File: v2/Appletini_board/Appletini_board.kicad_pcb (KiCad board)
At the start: 4 copper layers, 152.4 x 69.8 mm, 32 parts, among them J1 Conn_02x25_Counter_Clockwise, Q1 TP0610T, U1 SN74LVC543ADW, U10 SN74LVC543ADW, U14 74AHC1G126, U2 Pico, U3 Teensy4.1, U4 SN74LVC543ADW, U5 TXS0108EPW, U6 74LS08, U7 74AHC1G126, U8 SN74LVC1G14DBV, U9 SN74LVC543ADW

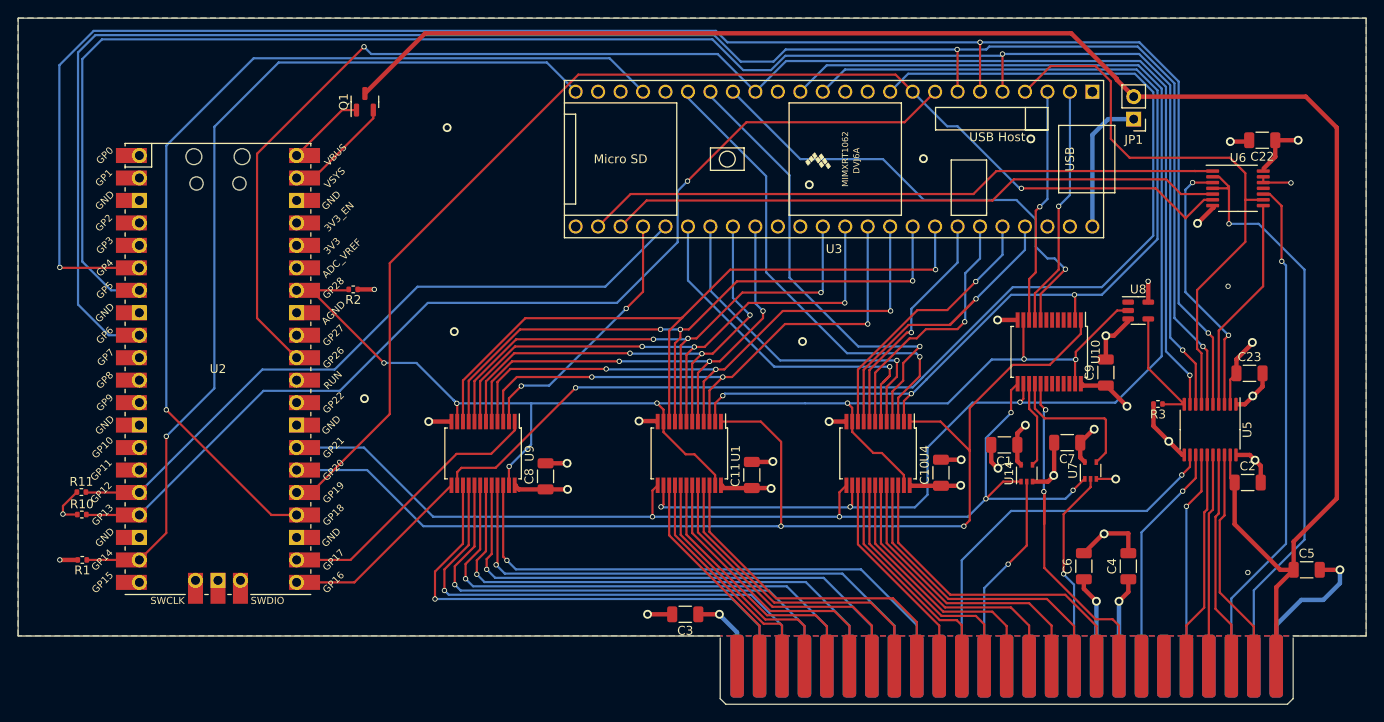
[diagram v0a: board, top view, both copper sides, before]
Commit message: fixes
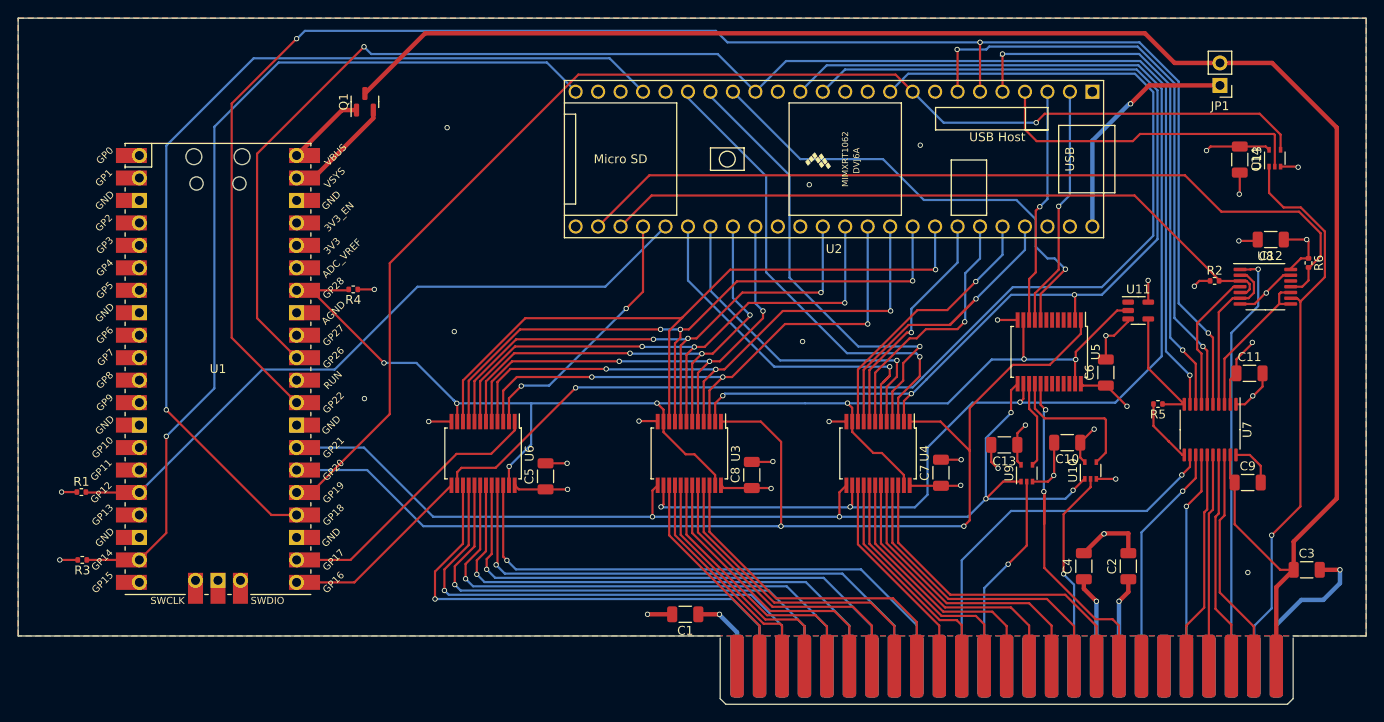
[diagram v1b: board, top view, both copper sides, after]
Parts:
- removed R10: 10K, Resistor_SMD:R_0402_1005Metric
- removed the U6 at (187.9, 69.2)
- added C14: 100pF, Capacitor_SMD:C_1206_3216Metric, F.Cu at (188.1, 66.0)
- added R2: 10K, Resistor_SMD:R_0402_1005Metric, F.Cu at (185.3, 79.7)
- added R6: 10K, Resistor_SMD:R_0402_1005Metric, F.Cu at (195.9, 77.7)
- added U13: 74LVC1G08, Package_TO_SOT_SMD:SOT-353_SC-70-5, F.Cu at (192.1, 65.8)
- added U8: 74LCX07, Package_SO:TSSOP-14_4.4x5mm_P0.65mm, F.Cu at (191.0, 80.4)
- moved C12 11.3 mm to (191.6, 75.0)
- moved JP1 10.5 mm to (185.9, 57.6)
- renumbered C3 to C1, C7 to C10, C23 to C11, C22 to C12, C1 to C13, C4 to C2, C5 to C3, C6 to C4, C8 to C5, C9 to C6, C10 to C7, C11 to C8, C2 to C9, R11 to R1, R1 to R3, R2 to R4, R3 to R5, U2 to U1, U7 to U10, U8 to U11, U3 to U2, U1 to U3, U10 to U5, U9 to U6, U5 to U7, U14 to U9
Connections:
- net /PICO_DMA_CYCLE renamed /DMA_CYCLE_ACTIVE
- net /PICO_TEENSY_~{IRQ} renamed /TEENSY_~{IRQ}
- U1 pad 13: unconnected-(U2-GND-Pad13) -> GND
- U1 pad 17: /TEENSY_~{INH} -> unconnected-(U1-GPIO13-Pad17)
- U1 pad 18: unconnected-(U2-GND-Pad18) -> GND
- U1 pad 23: unconnected-(U2-GND-Pad23) -> GND
- U1 pad 28: unconnected-(U2-GND-Pad28) -> GND
- U1 pad 29: unconnected-(U2-GPIO22-Pad29) -> /~{DMA}
- U1 pad 3: unconnected-(U2-GND-Pad3) -> GND
- U1 pad 33: unconnected-(U2-AGND-Pad33) -> GND
- U1 pad 38: unconnected-(U2-GND-Pad38) -> GND
- U1 pad 6: /PICO_CTRL_~{DMA} -> unconnected-(U1-GPIO4-Pad6)
- U1 pad 7: /PICO_CTRL_~{INH} -> unconnected-(U1-GPIO5-Pad7)
- U1 pad 8: unconnected-(U2-GND-Pad8) -> GND
- U1 pad 9: /PICO_CTRL_~{RDY} -> unconnected-(U1-GPIO6-Pad9)
- U2 pad 27: /TEENSY_REQ_DMA -> /TEENSY_REQ_~{IRQ}
- U2 pad 4: /TEENSY_CTRL_~{IRQ} -> /TEENSY_REQ_DMA
- U2 pad 5: /PICO_CTRL_~{INH} -> /~{INH}
- U2 pad 6: /PICO_CTRL_~{DMA} -> /~{DMA}
- U2 pad 7: /PICO_CTRL_~{RDY} -> /~{RDY}
- U2 pad 8: /TEENSY_~{INH} -> unconnected-(U2-GPIO7.10-Pad8)
- U7 pad 3: /Bus transceivers/CTRL_~{DMAOUT} -> /Bus transceivers/~{DMAOUT}
- U7 pad 4: /Bus transceivers/CTRL_~{INTOUT} -> /Bus transceivers/~{INTOUT}
- U7 pad 5: /PICO_CTRL_~{DMA} -> /~{DMA}
- U7 pad 6: /PICO_CTRL_~{RDY} -> /~{RDY}
- U7 pad 7: /TEENSY_CTRL_~{IRQ} -> /Bus transceivers/~{IRQ}
- U7 pad 8: /PICO_CTRL_~{INH} -> /~{INH}
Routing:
- net /PICO_CTRL_~{RDY}: track 207.9 -> 0.00 mm, vias 2 -> 0
- net /PICO_CTRL_~{DMA}: track 206.3 -> 0.00 mm, vias 3 -> 0
- net /PICO_CTRL_~{INH}: track 199.8 -> 0.00 mm, vias 2 -> 0
- net /~{DMA}: track 0.00 -> 193.5 mm, vias 0 -> 3
- net /TEENSY_~{INH}: track 119.2 -> 0.00 mm, vias 1 -> 0
- net /TEENSY_REQ_~{IRQ}: track 0.00 -> 78.6 mm
- net /~{RDY}: track 0.00 -> 69.0 mm, vias 0 -> 2
- net /TEENSY_CTRL_~{IRQ}: track 65.6 -> 0.00 mm
- net /~{INH}: track 0.00 -> 62.3 mm, vias 0 -> 2
- net /TEENSY_REQ_DMA: track 69.8 -> 37.7 mm
- net /Bus transceivers/CTRL_~{DMAOUT}: track 30.0 -> 0.00 mm, vias 2 -> 0
- net /Bus transceivers/CTRL_~{INTOUT}: track 24.6 -> 0.00 mm
- net /TEENSY_REQ_~{DMAOUT}: track 72.1 -> 95.1 mm
- net /Bus transceivers/~{INTOUT}: track 0.00 -> 18.4 mm
- net /Bus transceivers/~{DMAOUT}: track 0.00 -> 17.7 mm
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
